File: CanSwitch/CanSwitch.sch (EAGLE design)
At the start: 17 parts

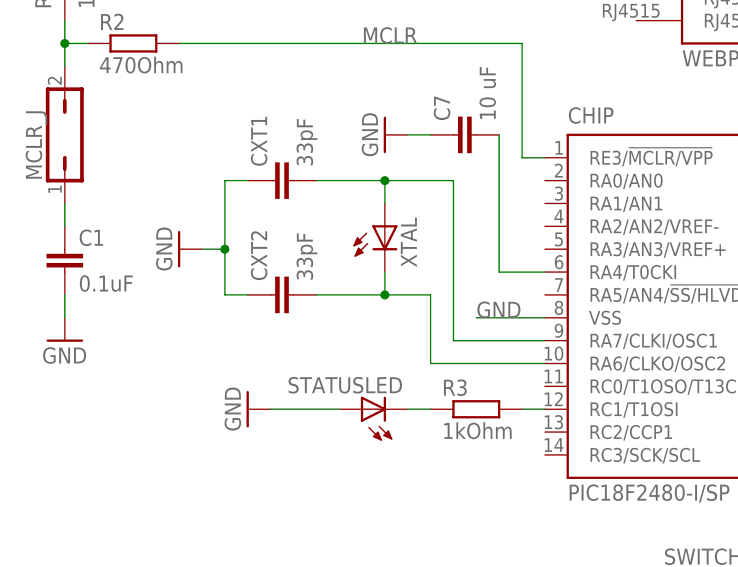
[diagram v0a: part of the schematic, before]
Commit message: first attempt to do proper wiring on the board
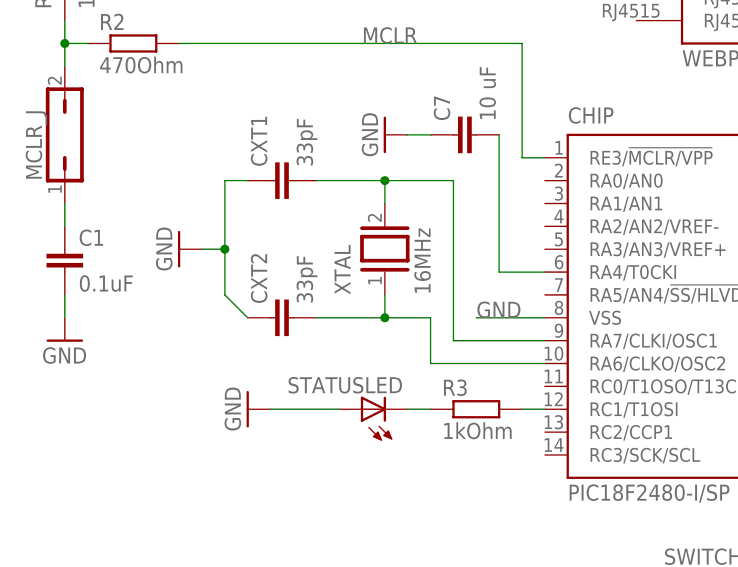
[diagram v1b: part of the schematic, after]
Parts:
- XTAL: value (none) -> 16MHz; device led:LED5MM -> special:XTAL/S
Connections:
- removed net N$5: CHIP.RA6/CLKO/OSC2, CXT2.2, XTAL.C
- new net N$3: CHIP.RA6/CLKO/OSC2, CXT2.2, XTAL.1
- net N$6: now also XTAL.2; no longer XTAL.A
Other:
- moved on the sheet: CXT2
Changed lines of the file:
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@@
 <part name="C7" library="rcl" deviceset="C-EU" device="C0805" value="10 uF"/>
 <part name="GND5" library="supply1" deviceset="GND" device=""/>
-<part name="XTAL" library="led" deviceset="LED" device="5MM"/>
 <part name="CXT1" library="rcl" deviceset="C-EU" device="C0805" value="33pF"/>
 <part name="CXT2" library="rcl" deviceset="C-EU" device="C0805" value="33pF"/>
@@
 <part name="GND3" library="supply1" deviceset="GND" device=""/>
 <part name="C3" library="rcl" deviceset="C-EU" device="C0805" value="0.1uF"/>
+<part name="XTAL" library="special" deviceset="XTAL/S" device="" value="16MHz"/>
 </parts>
 <sheets>
@@
 <instance part="C7" gate="G$1" x="-111.76" y="106.68" rot="R90"/>
 <instance part="GND5" gate="1" x="-119.38" y="106.68" rot="R270"/>
-<instance part="XTAL" gate="G$1" x="-119.38" y="96.52"/>
 <instance part="CXT1" gate="G$1" x="-132.08" y="101.6" rot="R90"/>
-<instance part="CXT2" gate="G$1" x="-132.08" y="88.9" rot="R90"/>
+<instance part="CXT2" gate="G$1" x="-132.08" y="86.36" rot="R90"/>
 <instance part="GND6" gate="1" x="-142.24" y="93.98" rot="R270"/>
 <instance part="R3" gate="G$1" x="-109.22" y="76.2"/>
@@
 <instance part="GND3" gate="1" x="-27.94" y="104.14" rot="R270"/>
 <instance part="C3" gate="G$1" x="-20.32" y="99.06"/>
+<instance part="XTAL" gate="G$1" x="-119.38" y="93.98" rot="R90"/>
 </instances>
 <busses>
@@
 <segment>
 <pinref part="CXT2" gate="G$1" pin="1"/>
-<wire x1="-134.62" y1="88.9" x2="-137.16" y2="88.9" width="0.1524" layer="91"/>
+<wire x1="-134.62" y1="86.36" x2="-137.16" y2="88.9" width="0.1524" layer="91"/>
 <wire x1="-137.16" y1="88.9" x2="-137.16" y2="93.98" width="0.1524" layer="91"/>
 <pinref part="GND6" gate="1" pin="GND"/>
@@
 <pinref part="CXT1" gate="G$1" pin="2"/>
 <wire x1="-111.76" y1="101.6" x2="-119.38" y2="101.6" width="0.1524" layer="91"/>
-<pinref part="XTAL" gate="G$1" pin="A"/>
+<pinref part="XTAL" gate="G$1" pin="2"/>
 <wire x1="-119.38" y1="101.6" x2="-127" y2="101.6" width="0.1524" layer="91"/>
 <wire x1="-119.38" y1="99.06" x2="-119.38" y2="101.6" width="0.1524" layer="91"/>
@@
 </segment>
 </net>
-<net name="N$5" class="0">
-<segment>
-<pinref part="CHIP" gate="G$1" pin="RA6/CLKO/OSC2"/>
-<wire x1="-101.6" y1="81.28" x2="-114.3" y2="81.28" width="0.1524" layer="91"/>
-<wire x1="-114.3" y1="81.28" x2="-114.3" y2="88.9" width="0.1524" layer="91"/>
-<pinref part="CXT2" gate="G$1" pin="2"/>
-<wire x1="-114.3" y1="88.9" x2="-119.38" y2="88.9" width="0.1524" layer="91"/>
-<pinref part="XTAL" gate="G$1" pin="C"/>
-<wire x1="-119.38" y1="88.9" x2="-127" y2="88.9" width="0.1524" layer="91"/>
-<wire x1="-119.38" y1="91.44" x2="-119.38" y2="88.9" width="0.1524" layer="91"/>
-<junction x="-119.38" y="88.9"/>
-</segment>
-</net>
 <net name="N$7" class="0">
 <segment>
@@
 </segment>
 </net>
+<net name="N$3" class="0">
+<segment>
+<pinref part="CHIP" gate="G$1" pin="RA6/CLKO/OSC2"/>
+<wire x1="-101.6" y1="81.28" x2="-114.3" y2="81.28" width="0.1524" layer="91"/>
+<wire x1="-114.3" y1="81.28" x2="-114.3" y2="86.36" width="0.1524" layer="91"/>
+<pinref part="CXT2" gate="G$1" pin="2"/>
+<wire x1="-114.3" y1="86.36" x2="-119.38" y2="86.36" width="0.1524" layer="91"/>
+<pinref part="XTAL" gate="G$1" pin="1"/>
+<wire x1="-119.38" y1="86.36" x2="-127" y2="86.36" width="0.1524" layer="91"/>
+<wire x1="-119.38" y1="88.9" x2="-119.38" y2="86.36" width="0.1524" layer="91"/>
+<junction x="-119.38" y="86.36"/>
+</segment>
+</net>
